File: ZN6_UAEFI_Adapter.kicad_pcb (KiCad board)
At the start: 2 copper layers, 148.3 x 160.6 mm, 22 parts, among them U1 ADS1015IDGS, U3 MIC5205-3.3YM5

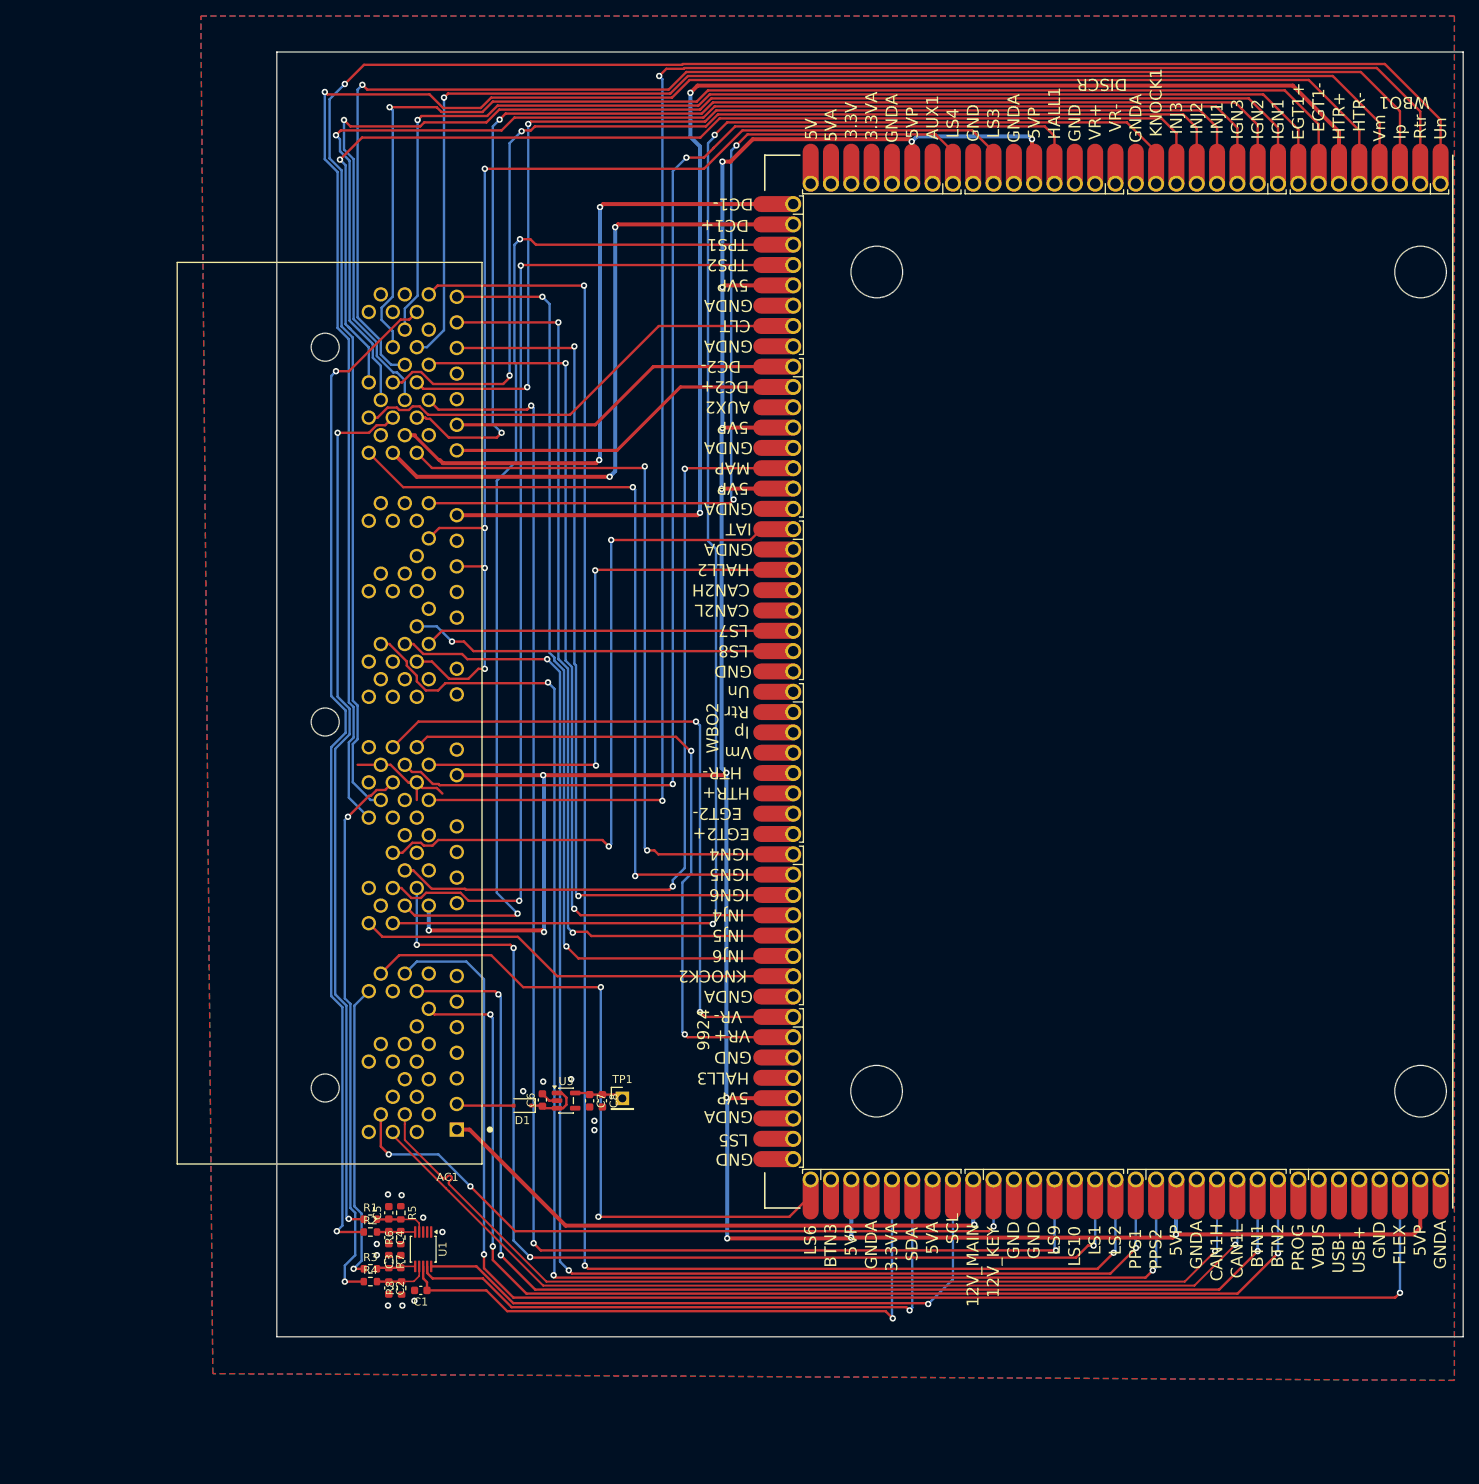
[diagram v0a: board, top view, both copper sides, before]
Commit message: First Draft of Adapter board
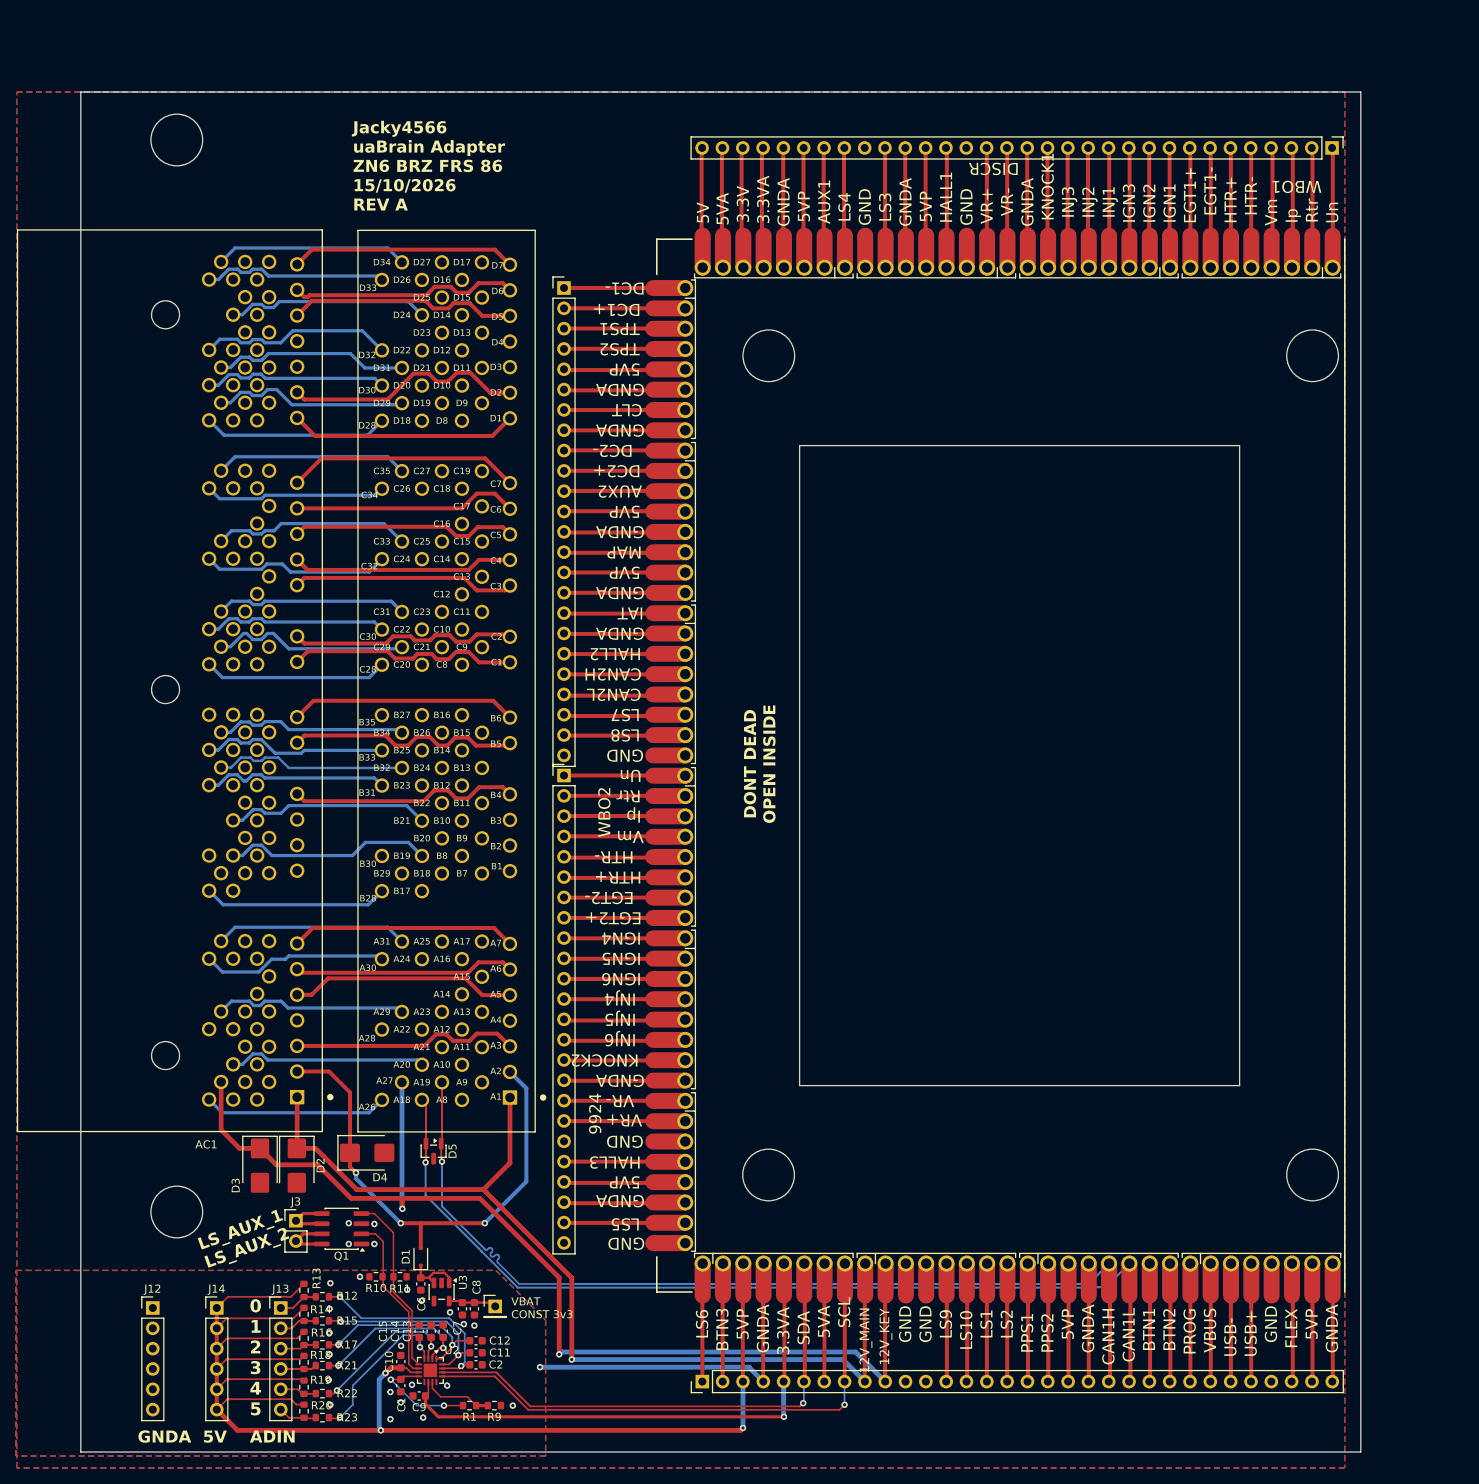
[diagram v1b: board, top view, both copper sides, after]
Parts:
- removed C3, C4, C5: 10nF, Capacitor_SMD:C_0603_1608Metric
- removed R2, R3, R4: 10k, Resistor_SMD:R_0603_1608Metric
- removed R5, R6, R7, R8: 20k, Resistor_SMD:R_0603_1608Metric
- removed U1: ADS1015IDGS, Package_SO:TSSOP-10_3x3mm_P0.5mm
- added AC2: 6376430-2, ZN6:TE_6376430-2, F.Cu at (86.6, 176.0)
- added C10: 1uF, Capacitor_SMD:C_0603_1608Metric, F.Cu at (84.0, 208.7)
- added C11: 10nF, Capacitor_SMD:C_0603_1608Metric, F.Cu at (93.4, 207.6)
- added C12: 10nF, Capacitor_SMD:C_0603_1608Metric, F.Cu at (93.4, 206.1)
- added C13: 10nF, Capacitor_SMD:C_0603_1608Metric, F.Cu at (89.3, 204.9)
- added C14: 10nF, Capacitor_SMD:C_0603_1608Metric, F.Cu at (87.8, 204.9)
- added C15: 10nF, Capacitor_SMD:C_0603_1608Metric, F.Cu at (86.3, 204.9)
- added C9: 1uF, Capacitor_SMD:C_0603_1608Metric, F.Cu at (86.3, 213.0)
- added D2: SMBJ24A, Diode_SMD:D_SMB, F.Cu at (71.0, 184.2)
- added D3: SMBJ24A, Diode_SMD:D_SMB, F.Cu at (66.4, 184.2)
- added D4: SMBJ24A, Diode_SMD:D_SMB, F.Cu at (79.8, 182.6)
- added D5: SZNUP2105L, Package_TO_SOT_SMD:SOT-23, F.Cu at (88.1, 182.4)
- added J1: Conn_01x32_Socket, Connector_PinHeader_2.54mm:PinHeader_1x32_P2.54mm_Vertical, F.Cu at (200.4, 57.0)
- added J12: Conn_01x06_Socket, Connector_PinHeader_2.54mm:PinHeader_1x06_P2.54mm_Vertical, F.Cu at (53.0, 202.0)
- added J13: Conn_01x06_Socket, Connector_PinHeader_2.54mm:PinHeader_1x06_P2.54mm_Vertical, F.Cu at (69.0, 202.0)
- added J14: Conn_01x06_Socket, Connector_PinHeader_2.54mm:PinHeader_1x06_P2.54mm_Vertical, F.Cu at (61.0, 202.0)
- added J2: Conn_01x32_Socket, Connector_PinHeader_2.54mm:PinHeader_1x32_P2.54mm_Vertical, F.Cu at (121.7, 211.2)
- added J3: Conn_01x02_Socket, Connector_PinHeader_2.54mm:PinHeader_1x02_P2.54mm_Vertical, F.Cu at (70.9, 191.1)
- added J4: Conn_01x24_Socket, Connector_PinHeader_2.54mm:PinHeader_1x24_P2.54mm_Vertical, F.Cu at (104.4, 74.5)
- added J5: Conn_01x24_Socket, Connector_PinHeader_2.54mm:PinHeader_1x24_P2.54mm_Vertical, F.Cu at (104.4, 135.4)
- added Q1: NCV8402ADDR2G, Package_SO:SOIC-8_3.9x4.9mm_P1.27mm, F.Cu at (76.6, 192.1)
- added R10: 10k, Resistor_SMD:R_0603_1608Metric, F.Cu at (80.9, 198.1)
- added R11: 10k, Resistor_SMD:R_0603_1608Metric, F.Cu at (83.9, 198.1)
- added R12: 4.7k, Resistor_SMD:R_0603_1608Metric, F.Cu at (74.2, 200.6)
- added R13: 10k, Resistor_SMD:R_0603_1608Metric, F.Cu at (71.9, 199.8)
- added R14: 10k, Resistor_SMD:R_0603_1608Metric, F.Cu at (71.9, 202.8)
- added R15: 4.7k, Resistor_SMD:R_0603_1608Metric, F.Cu at (74.2, 203.6)
- added R16: 10k, Resistor_SMD:R_0603_1608Metric, F.Cu at (71.9, 205.8)
- added R17: 4.7k, Resistor_SMD:R_0603_1608Metric, F.Cu at (74.2, 206.6)
- added R18: 10k, Resistor_SMD:R_0603_1608Metric, F.Cu at (71.9, 208.8)
- added R19: 10k, Resistor_SMD:R_0603_1608Metric, F.Cu at (71.9, 211.9)
- added R20: 10k, Resistor_SMD:R_0603_1608Metric, F.Cu at (71.9, 214.9)
- added R21: 4.7k, Resistor_SMD:R_0603_1608Metric, F.Cu at (74.2, 209.2)
- added R22: 4.7k, Resistor_SMD:R_0603_1608Metric, F.Cu at (74.2, 212.7)
- added R23: 4.7k, Resistor_SMD:R_0603_1608Metric, F.Cu at (74.2, 215.7)
- added R9: DNP, Resistor_SMD:R_0603_1608Metric, F.Cu at (95.7, 214.2)
- added U2: ADS7128IRTER, Package_DFN_QFN:WQFN-16-1EP_3x3mm_P0.5mm_EP1.68x1.68mm, F.Cu at (87.7, 209.8)
- R1: value 10k -> 11k
- moved C8 30.5 mm to (93.2, 202.1)
- moved TP1 30.5 mm to (95.8, 201.8)
- moved C7 30.5 mm to (91.7, 202.1)
- moved U3 28.5 mm to (89.1, 200.0), turned to -90 degrees
- moved C6 27.6 mm to (86.5, 199.0), turned to -90 degrees
- moved R1 26.4 mm to (92.6, 214.2), turned to 180 degrees
- moved D1 22.8 mm to (86.5, 195.6), turned to 90 degrees
- moved AC1 20.4 mm to (60.0, 175.9)
- moved hw-uaBrain1 17.1 mm to (202.0, 200.0)
- moved C2 14.5 mm to (93.4, 209.1), turned to 0 degrees
- moved C1 12.2 mm to (84.0, 211.7), turned to -90 degrees
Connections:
- AC1 pad 10: unconnected-(AC1-Pad10) -> Net-(AC1-Pad10)
- AC1 pad 100: unconnected-(AC1-Pad100) -> Net-(AC1-Pad100)
- AC1 pad 101: unconnected-(AC1-Pad101) -> Net-(AC1-Pad101)
- AC1 pad 102: /OUT_DC2+ -> Net-(AC1-Pad102)
- AC1 pad 103: /OUT_DC2- -> Net-(AC1-Pad103)
- AC1 pad 104: unconnected-(AC1-Pad104) -> GND
- AC1 pad 106: /OUT_IGN6 -> Net-(AC1-Pad106)
- AC1 pad 107: /OUT_INJ5 -> Net-(AC1-Pad107)
- AC1 pad 108: /OUT_INJ6 -> Net-(AC1-Pad108)
- AC1 pad 109: /OUT_IGN4 -> Net-(AC1-Pad109)
- AC1 pad 11: unconnected-(AC1-Pad11) -> Net-(AC1-Pad11)
- AC1 pad 110: unconnected-(AC1-Pad110) -> Net-(AC1-Pad110)
- AC1 pad 111: /OUT_IGN2 -> Net-(AC1-Pad111)
- AC1 pad 112: /PURGE_VALVE -> Net-(AC1-Pad112)
- AC1 pad 113: /OUT_INJ1 -> Net-(AC1-Pad113)
- AC1 pad 114: /OUT_INJ4 -> Net-(AC1-Pad114)
- AC1 pad 115: /2_WBO1_Vm -> Net-(AC1-Pad115)
- AC1 pad 116: unconnected-(AC1-Pad116) -> Net-(AC1-Pad116)
- AC1 pad 117: /OIL_PRESSURE -> Net-(AC1-Pad117)
- AC1 pad 118: /VVT Inlet Solenoid LH -> Net-(AC1-Pad118)
- AC1 pad 119: /OUT_DC1+ -> Net-(AC1-Pad119)
- AC1 pad 12: unconnected-(AC1-Pad12) -> Net-(AC1-Pad12)
- AC1 pad 120: /OUT_DC1- -> Net-(AC1-Pad120)
- AC1 pad 121: /OIL_TEMP -> Net-(AC1-Pad121)
- AC1 pad 122: /OUT_IGN1 -> Net-(AC1-Pad122)
- AC1 pad 123: /OUT_INJ2 -> Net-(AC1-Pad123)
- AC1 pad 124: /1_WBO1_Ip -> Net-(AC1-Pad124)
- AC1 pad 125: /EGT1- -> Net-(AC1-Pad125)
- AC1 pad 126: /EGT1+ -> Net-(AC1-Pad126)
- AC1 pad 127: unconnected-(AC1-Pad127) -> Net-(AC1-Pad127)
- AC1 pad 128: unconnected-(AC1-Pad128) -> Net-(AC1-Pad128)
- AC1 pad 129: /OUT_IGN5 -> Net-(AC1-Pad129)
- AC1 pad 13: unconnected-(AC1-Pad13) -> Net-(AC1-Pad13)
- AC1 pad 130: GND -> Net-(AC1-Pad130)
- AC1 pad 131: /IN_CLT -> Net-(AC1-Pad131)
- AC1 pad 132: /OUT_IGN3 -> Net-(AC1-Pad132)
- AC1 pad 133: /OUT_INJ3 -> Net-(AC1-Pad133)
- AC1 pad 134: unconnected-(AC1-Pad134) -> Net-(AC1-Pad134)
- AC1 pad 135: unconnected-(AC1-Pad135) -> Net-(AC1-Pad135)
- AC1 pad 14: unconnected-(AC1-Pad14) -> Net-(AC1-Pad14)
- AC1 pad 15: /CLUTCH_SW -> Net-(AC1-Pad15)
- AC1 pad 16: /NSW -> Net-(AC1-Pad16)
- AC1 pad 17: unconnected-(AC1-Pad17) -> Net-(AC1-Pad17)
- AC1 pad 20: unconnected-(AC1-Pad20) -> Net-(AC1-Pad20)
- AC1 pad 21: unconnected-(AC1-Pad21) -> Net-(AC1-Pad21)
- AC1 pad 22: GND -> Net-(AC1-Pad22)
- AC1 pad 23: unconnected-(AC1-Pad23) -> Net-(AC1-Pad23)
- AC1 pad 24: unconnected-(AC1-Pad24) -> Net-(AC1-Pad24)
- AC1 pad 25: /IN_FLEX -> Net-(AC1-Pad25)
- AC1 pad 26: unconnected-(AC1-Pad26) -> Net-(AC1-Pad26)
- AC1 pad 29: unconnected-(AC1-Pad29) -> Net-(AC1-Pad29)
- AC1 pad 3: unconnected-(AC1-Pad3) -> Net-(AC1-Pad3)
- AC1 pad 30: /CRUISE_CCS -> Net-(AC1-Pad30)
- AC1 pad 31: /Oil_Pressure_Dash -> Net-(AC1-Pad31)
- AC1 pad 35: unconnected-(AC1-Pad35) -> Net-(AC1-Pad35)
- AC1 pad 36: /+5VP -> Net-(AC1-Pad36)
- AC1 pad 37: unconnected-(AC1-Pad37) -> Net-(AC1-Pad37)
- AC1 pad 38: /+5VP -> Net-(AC1-Pad38)
- AC1 pad 39: /VVT Inlet Solenoid RH -> Net-(AC1-Pad39)
- AC1 pad 4: unconnected-(AC1-Pad4) -> GND
- AC1 pad 40: GND -> Net-(AC1-Pad40)
- AC1 pad 41: unconnected-(AC1-Pad41) -> Net-(AC1-Pad41)
- AC1 pad 42: unconnected-(AC1-Pad42) -> Net-(AC1-Pad42)
- AC1 pad 43: unconnected-(AC1-Pad43) -> Net-(AC1-Pad43)
- AC1 pad 44: /5_WBO1_Rtrim -> Net-(AC1-Pad44)
- AC1 pad 45: GND -> Net-(AC1-Pad45)
- AC1 pad 46: /VVT Inlet Sensor LH -> Net-(AC1-Pad46)
- AC1 pad 47: /CRANK_VR+ -> Net-(AC1-Pad47)
- AC1 pad 48: /IN_KNOCK1_RAW -> Net-(AC1-Pad48)
- AC1 pad 49: /IN_TPS1 -> Net-(AC1-Pad49)
- AC1 pad 5: unconnected-(AC1-Pad5) -> Net-(AC1-Pad5)
- AC1 pad 50: /IN_TPS2 -> Net-(AC1-Pad50)
- AC1 pad 51: /IN_MAP -> Net-(AC1-Pad51)
- AC1 pad 52: /IN_IAT -> Net-(AC1-Pad52)
- AC1 pad 53: unconnected-(AC1-Pad53) -> Net-(AC1-Pad53)
- AC1 pad 54: unconnected-(AC1-Pad54) -> Net-(AC1-Pad54)
- AC1 pad 55: unconnected-(AC1-Pad55) -> Net-(AC1-Pad55)
- AC1 pad 56: /FUEL_PRESSURE -> Net-(AC1-Pad56)
- AC1 pad 57: /VVT Inlet Sensor RH -> Net-(AC1-Pad57)
- AC1 pad 58: /CRANK_VR- -> Net-(AC1-Pad58)
- AC1 pad 59: /IN_KNOCK2_RAW -> Net-(AC1-Pad59)
- AC1 pad 6: unconnected-(AC1-Pad6) -> Net-(AC1-Pad6)
- AC1 pad 60: unconnected-(AC1-Pad60) -> GND
- AC1 pad 61: unconnected-(AC1-Pad61) -> GND
- AC1 pad 62: /3_WBO1_Heater -> Net-(AC1-Pad62)
- AC1 pad 63: /6_WBO1_Un -> Net-(AC1-Pad63)
- AC1 pad 64: unconnected-(AC1-Pad64) -> Net-(AC1-Pad64)
- AC1 pad 65: GND -> Net-(AC1-Pad65)
- AC1 pad 66: unconnected-(AC1-Pad66) -> GND
- AC1 pad 67: unconnected-(AC1-Pad67) -> Net-(AC1-Pad67)
- AC1 pad 68: unconnected-(AC1-Pad68) -> Net-(AC1-Pad68)
- AC1 pad 69: unconnected-(AC1-Pad69) -> Net-(AC1-Pad69)
- AC1 pad 7: /BRAKE_SW -> Net-(AC1-Pad7)
- AC1 pad 70: unconnected-(AC1-Pad70) -> Net-(AC1-Pad70)
- AC1 pad 71: /ETCS_RELAY -> Net-(AC1-Pad71)
- AC1 pad 72: unconnected-(AC1-Pad72) -> Net-(AC1-Pad72)
- AC1 pad 73: /+12V_RAW_FROM_ETCS -> Net-(AC1-Pad73)
- AC1 pad 74: unconnected-(AC1-Pad74) -> Net-(AC1-Pad74)
- AC1 pad 75: unconnected-(AC1-Pad75) -> Net-(AC1-Pad75)
- AC1 pad 76: /ETCS_RELAY -> Net-(AC1-Pad76)
- AC1 pad 77: /FAN1 -> Net-(AC1-Pad77)
- AC1 pad 78: /FAN2 -> Net-(AC1-Pad78)
- AC1 pad 79: /EFI_RELAYS -> Net-(AC1-Pad79)
- AC1 pad 8: unconnected-(AC1-Pad8) -> Net-(AC1-Pad8)
- AC1 pad 80: unconnected-(AC1-Pad80) -> Net-(AC1-Pad80)
- AC1 pad 81: unconnected-(AC1-Pad81) -> Net-(AC1-Pad81)
- AC1 pad 82: unconnected-(AC1-Pad82) -> Net-(AC1-Pad82)
- AC1 pad 83: /ETCS_RELAY -> Net-(AC1-Pad83)
- AC1 pad 84: unconnected-(AC1-Pad84) -> Net-(AC1-Pad84)
- AC1 pad 85: /FP_CONTROL -> Net-(AC1-Pad85)
- AC1 pad 86: unconnected-(AC1-Pad86) -> Net-(AC1-Pad86)
- AC1 pad 87: unconnected-(AC1-Pad87) -> Net-(AC1-Pad87)
- AC1 pad 88: unconnected-(AC1-Pad88) -> Net-(AC1-Pad88)
- AC1 pad 89: /IN_PPS1 -> Net-(AC1-Pad89)
- AC1 pad 9: unconnected-(AC1-Pad9) -> Net-(AC1-Pad9)
- AC1 pad 90: unconnected-(AC1-Pad90) -> Net-(AC1-Pad90)
- AC1 pad 91: unconnected-(AC1-Pad91) -> Net-(AC1-Pad91)
- AC1 pad 92: unconnected-(AC1-Pad92) -> Net-(AC1-Pad92)
- AC1 pad 93: unconnected-(AC1-Pad93) -> Net-(AC1-Pad93)
- AC1 pad 94: unconnected-(AC1-Pad94) -> Net-(AC1-Pad94)
- AC1 pad 95: GND -> Net-(AC1-Pad95)
- AC1 pad 96: GND -> Net-(AC1-Pad96)
- AC1 pad 97: /IN_PPS2 -> Net-(AC1-Pad97)
- AC1 pad 98: unconnected-(AC1-Pad98) -> Net-(AC1-Pad98)
- AC1 pad 99: unconnected-(AC1-Pad99) -> Net-(AC1-Pad99)
- C1 pad 1: /+3.3VA -> /ADS712/ADS_DECAP
- C1 pad 2: GND -> GNDA
- C2 pad 1: Net-(U1-AIN3) -> /ADS712/AIN0
- C2 pad 2: GND -> GNDA
- C6 pad 2: GND -> GNDA
- C7 pad 2: GND -> GNDA
- C8 pad 2: GND -> GNDA
- R1 pad 1: /OIL_TEMP -> Net-(U2-ADDR)
- R1 pad 2: Net-(U1-AIN0) -> /ADS712/ADS_DECAP
- U3 pad 2: GND -> GNDA
- hw-uaBrain1 pad A1: /6_WBO1_Un -> Net-(J1-Pin_1)
- hw-uaBrain1 pad A2: /5_WBO1_Rtrim -> Net-(J1-Pin_2)
- hw-uaBrain1 pad A3: /1_WBO1_Ip -> Net-(J1-Pin_3)
- hw-uaBrain1 pad A4: /2_WBO1_Vm -> Net-(J1-Pin_4)
- hw-uaBrain1 pad A5: /3_WBO1_Heater -> Net-(J1-Pin_5)
- hw-uaBrain1 pad A6: /+12V_RAW_FROM_ETCS -> Net-(J1-Pin_6)
- hw-uaBrain1 pad A7: /EGT1- -> Net-(J1-Pin_7)
- hw-uaBrain1 pad A8: /EGT1+ -> Net-(J1-Pin_8)
- hw-uaBrain1 pad B1: /OUT_IGN1 -> Net-(J1-Pin_9)
- hw-uaBrain1 pad B2: /OUT_IGN2 -> Net-(J1-Pin_10)
- hw-uaBrain1 pad B3: /OUT_IGN3 -> Net-(J1-Pin_11)
- hw-uaBrain1 pad B4: /OUT_INJ1 -> Net-(J1-Pin_12)
- hw-uaBrain1 pad B5: /OUT_INJ2 -> Net-(J1-Pin_13)
- hw-uaBrain1 pad B6: /OUT_INJ3 -> Net-(J1-Pin_14)
- hw-uaBrain1 pad B7: /IN_KNOCK1_RAW -> Net-(J1-Pin_15)
- hw-uaBrain1 pad B8: GND -> Net-(J1-Pin_16)
- hw-uaBrain1 pad C1: unconnected-(hw-uaBrain1A-VR_DISCRETE--PadC1)_1 -> Net-(J1-Pin_17)
- hw-uaBrain1 pad C2: unconnected-(hw-uaBrain1A-VR_DISCRETE+-PadC2) -> Net-(J1-Pin_18)
- hw-uaBrain1 pad C4: /VVT Inlet Sensor RH -> Net-(J1-Pin_20)
- hw-uaBrain1 pad C5: /+5VP -> Net-(J1-Pin_21)
- hw-uaBrain1 pad C6: GND -> Net-(J1-Pin_22)
- hw-uaBrain1 pad C7: /ETCS_RELAY -> Net-(J1-Pin_23)
- hw-uaBrain1 pad D1: /FP_CONTROL -> Net-(J1-Pin_25)
- hw-uaBrain1 pad D2: unconnected-(hw-uaBrain1A-IN_AUX1-PadD2)_1 -> Net-(J1-Pin_26)
- hw-uaBrain1 pad D3: /+5VP -> Net-(J1-Pin_27)
- hw-uaBrain1 pad D4: GND -> Net-(J1-Pin_28)
- hw-uaBrain1 pad D5: /+3.3VA -> Net-(J1-Pin_29)
- hw-uaBrain1 pad D6: /+3.3V -> Net-(J1-Pin_30)
- hw-uaBrain1 pad D7: /+5VA -> Net-(J1-Pin_31)
- hw-uaBrain1 pad D8: /+5V -> Net-(J1-Pin_32)
- hw-uaBrain1 pad E1: /OUT_DC1- -> Net-(J4-Pin_1)
- hw-uaBrain1 pad E2: /OUT_DC1+ -> Net-(J4-Pin_2)
- hw-uaBrain1 pad E3: /IN_TPS1 -> Net-(J4-Pin_3)
- hw-uaBrain1 pad E4: /IN_TPS2 -> Net-(J4-Pin_4)
- hw-uaBrain1 pad E5: /+5VP -> Net-(J4-Pin_5)
- hw-uaBrain1 pad E6: GND -> Net-(J4-Pin_6)
- hw-uaBrain1 pad E7: /IN_CLT -> Net-(J4-Pin_7)
- hw-uaBrain1 pad E8: GND -> Net-(J4-Pin_8)
- hw-uaBrain1 pad F1: /OUT_DC2- -> Net-(J4-Pin_9)
- hw-uaBrain1 pad F2: /OUT_DC2+ -> Net-(J4-Pin_10)
- hw-uaBrain1 pad F3: unconnected-(hw-uaBrain1B-IN_AUX2-PadF3) -> Net-(J4-Pin_11)
- hw-uaBrain1 pad F4: /+5VP -> Net-(J4-Pin_12)
- hw-uaBrain1 pad F5: GND -> Net-(J4-Pin_13)
- hw-uaBrain1 pad F6: /IN_MAP -> Net-(J4-Pin_14)
- hw-uaBrain1 pad F7: /+5VP -> Net-(J4-Pin_15)
- hw-uaBrain1 pad F8: GND -> Net-(J4-Pin_16)
- hw-uaBrain1 pad G1: /IN_IAT -> Net-(J4-Pin_17)
- hw-uaBrain1 pad G2: GND -> Net-(J4-Pin_18)
- hw-uaBrain1 pad G3: /VVT Inlet Sensor LH -> Net-(J4-Pin_19)
- hw-uaBrain1 pad G4: unconnected-(hw-uaBrain1B-CAN2+-PadG4) -> Net-(J4-Pin_20)
- hw-uaBrain1 pad G5: unconnected-(hw-uaBrain1B-CAN2--PadG5) -> Net-(J4-Pin_21)
- hw-uaBrain1 pad G6: /FAN1 -> Net-(J4-Pin_22)
- hw-uaBrain1 pad G7: /FAN2 -> Net-(J4-Pin_23)
- hw-uaBrain1 pad H1: unconnected-(hw-uaBrain1B-6_WBO2_Un-PadH1) -> Net-(J5-Pin_1)
- hw-uaBrain1 pad H2: unconnected-(hw-uaBrain1B-5_WBO2_Rtrim-PadH2)_1 -> Net-(J5-Pin_2)
- hw-uaBrain1 pad H3: unconnected-(hw-uaBrain1B-1_WBO2_Ip-PadH3)_1 -> Net-(J5-Pin_3)
- hw-uaBrain1 pad H4: unconnected-(hw-uaBrain1B-2_WBO2_Vm-PadH4)_1 -> Net-(J5-Pin_4)
- hw-uaBrain1 pad H5: unconnected-(hw-uaBrain1B-3_WBO2_Heater-PadH5)_1 -> Net-(J5-Pin_5)
- hw-uaBrain1 pad H6: unconnected-(hw-uaBrain1B-+12V_RAW-PadH6) -> Net-(J5-Pin_6)
- hw-uaBrain1 pad H7: unconnected-(hw-uaBrain1B-EGT2--PadH7)_1 -> Net-(J5-Pin_7)
- hw-uaBrain1 pad H8: unconnected-(hw-uaBrain1B-EGT2+-PadH8)_1 -> Net-(J5-Pin_8)
- hw-uaBrain1 pad J1: /OUT_IGN4 -> Net-(J5-Pin_9)
- hw-uaBrain1 pad J2: /OUT_IGN5 -> Net-(J5-Pin_10)
- hw-uaBrain1 pad J3: /OUT_IGN6 -> Net-(J5-Pin_11)
- hw-uaBrain1 pad J4: /OUT_INJ4 -> Net-(J5-Pin_12)
- hw-uaBrain1 pad J5: /OUT_INJ5 -> Net-(J5-Pin_13)
- hw-uaBrain1 pad J6: /OUT_INJ6 -> Net-(J5-Pin_14)
- hw-uaBrain1 pad J7: /IN_KNOCK2_RAW -> Net-(J5-Pin_15)
- hw-uaBrain1 pad J8: GND -> Net-(J5-Pin_16)
- hw-uaBrain1 pad K1: /CRANK_VR- -> Net-(J5-Pin_17)
- hw-uaBrain1 pad K2: /CRANK_VR+ -> Net-(J5-Pin_18)
- hw-uaBrain1 pad K4: unconnected-(hw-uaBrain1B-IN_HALL3-PadK4)_1 -> Net-(J5-Pin_20)
- hw-uaBrain1 pad K5: /+5VP -> Net-(J5-Pin_21)
- hw-uaBrain1 pad K6: GND -> Net-(J5-Pin_22)
- hw-uaBrain1 pad K7: /OUT_LS5 -> Net-(J5-Pin_23)
- hw-uaBrain1 pad L1: /Oil_Pressure_Dash -> Net-(J2-Pin_1)
- hw-uaBrain1 pad L2: /IN_BUTTON3 -> Net-(J2-Pin_2)
- hw-uaBrain1 pad L3: /+5VP -> /5VP
- hw-uaBrain1 pad L4: GND -> GNDA
- hw-uaBrain1 pad L7: /+5VA -> Net-(J2-Pin_7)
- hw-uaBrain1 pad M5: /PURGE_VALVE -> Net-(J2-Pin_13)
- hw-uaBrain1 pad M6: unconnected-(hw-uaBrain1C-OUT_LS10-PadM6)_1 -> Net-(J2-Pin_14)
- hw-uaBrain1 pad M7: /VVT Inlet Solenoid RH -> Net-(J2-Pin_15)
- hw-uaBrain1 pad M8: /VVT Inlet Solenoid LH -> Net-(J2-Pin_16)
- hw-uaBrain1 pad N1: /IN_PPS1 -> Net-(J2-Pin_17)
- hw-uaBrain1 pad N2: /IN_PPS2 -> Net-(J2-Pin_18)
- hw-uaBrain1 pad N3: /+5VP -> Net-(J2-Pin_19)
- hw-uaBrain1 pad N4: GND -> Net-(J2-Pin_20)
- hw-uaBrain1 pad N7: /NSW -> Net-(J2-Pin_23)
- hw-uaBrain1 pad N8: /CLUTCH_SW -> Net-(J2-Pin_24)
- hw-uaBrain1 pad P1: unconnected-(hw-uaBrain1C-PROG_BUTTON-PadP1)_1 -> Net-(J2-Pin_25)
- hw-uaBrain1 pad P2: unconnected-(hw-uaBrain1C-VBUS-PadP2) -> Net-(J2-Pin_26)
- hw-uaBrain1 pad P3: unconnected-(hw-uaBrain1C-USB--PadP3) -> Net-(J2-Pin_27)
- hw-uaBrain1 pad P4: unconnected-(hw-uaBrain1C-USB+-PadP4)_1 -> Net-(J2-Pin_28)
- hw-uaBrain1 pad P6: /IN_FLEX -> Net-(J2-Pin_30)
- hw-uaBrain1 pad P7: /+5VP -> Net-(J2-Pin_31)
- hw-uaBrain1 pad P8: GND -> Net-(J2-Pin_32)
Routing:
- net /+5VP: track 388.0 -> 0.00 mm, vias 14 -> 0
- net /6_WBO1_Un: track 241.1 -> 0.00 mm, vias 1 -> 0
- net /3_WBO1_Heater: track 232.3 -> 0.00 mm, vias 1 -> 0
- net /5_WBO1_Rtrim: track 224.8 -> 0.00 mm, vias 2 -> 0
- net /VVT Inlet Solenoid LH: track 218.7 -> 0.00 mm, vias 3 -> 0
- net /IN_KNOCK1_RAW: track 198.9 -> 0.00 mm, vias 2 -> 0
- net /PURGE_VALVE: track 192.9 -> 0.00 mm, vias 3 -> 0
- net /IN_PPS2: track 186.0 -> 0.00 mm, vias 3 -> 0
- net /5VP: track 0.00 -> 181.5 mm, vias 0 -> 3
- net /IN_FLEX: track 181.4 -> 0.00 mm, vias 2 -> 0
- net /IN_PPS1: track 177.1 -> 0.00 mm, vias 3 -> 0
- net /1_WBO1_Ip: track 176.9 -> 0.00 mm, vias 1 -> 0
- net /+12V_RAW_FROM_ETCS: track 171.8 -> 0.00 mm, vias 2 -> 0
- net /VVT Inlet Sensor RH: track 165.7 -> 0.00 mm, vias 2 -> 0
- net /OUT_IGN1: track 163.5 -> 0.00 mm, vias 1 -> 0
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- added copper zone on In1.Cu, net GND
- added copper zone on In2.Cu, net GND
- added copper zone on B.Cu, net GNDA
- added copper zone on F.Cu, net GNDA
- added copper zone on In1.Cu, net GNDA
- added copper zone on In2.Cu, net GNDA
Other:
- board size 148.3 x 160.6 mm -> 160 x 170 mm
- copper layers 2 -> 4
- board text added: "0 1 2 3 4 5"
- board text added: "DONT DEAD OPEN INSIDE"
- board text added: "GNDA 5V ADIN"
- board text added: "Jacky4566 uaBrain Adapter ZN6 BRZ FRS 86 15/10/2026 REV A"
- board text added: "LS_AUX_1 LS_AUX_2"
- board text added: "VBAT CONST 3v3"
